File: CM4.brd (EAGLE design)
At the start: 116.8 x 61.4 mm, 7 parts, among them J1 MAGJACK, J2 67800-5001, J3 RASPBERRYPI-40-PIN-GPIO_PTH_N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, J4 67800-5001, J5 67800-5001, J6 67800-5001

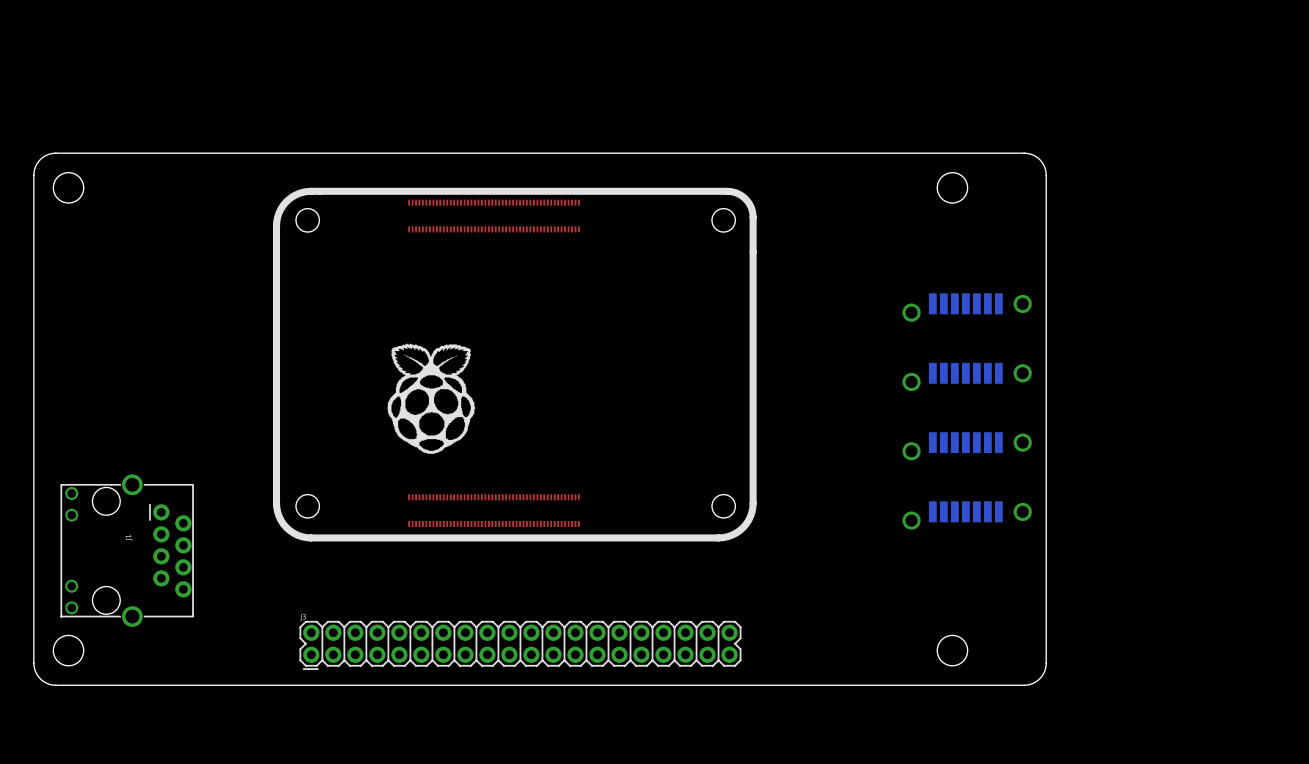
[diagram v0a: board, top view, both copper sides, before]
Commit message: finished board
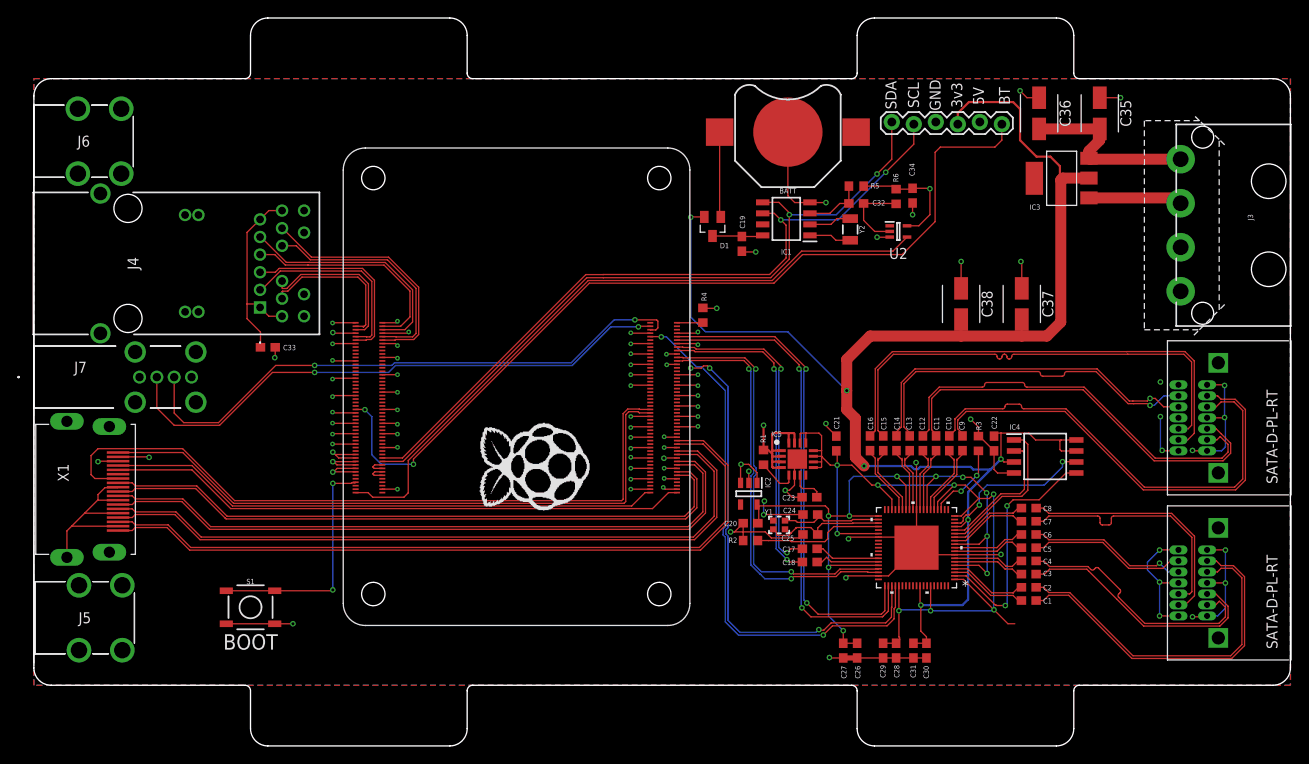
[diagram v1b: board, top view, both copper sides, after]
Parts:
- removed J2: 67800-5001, SamacSys_Parts:67800-5005_2
- added BATT: (no value), SparkFun-Batteries:BATTCON_12MM
- added C1, C10, C11, C12, C13, C14, C15, C16, C17, C18, C19, C2, C22, C3, C32, C33, C34, C4, C5, C6, C7, C8, C9: 0.1uF, SparkFun-Capacitors:0603
- added C20, C26, C28, C30: 1uF, SparkFun-Capacitors:0603
- added C21: 4.7uF, SparkFun-Capacitors:0603
- added C23: 10nF, SparkFun-Capacitors:0603
- added C24, C25: 18pF, SparkFun-Capacitors:0603
- added C27, C29, C31: 2.2uF, SparkFun-Capacitors:0603
- added C35, C36, C37, C38: 865080640004, SamacSys_Parts:865080640004
- added D1: BAT54C, diode:SOT23
- added IC1: PCF85063AT_AAZ, SamacSys_Parts:SOIC127P600X175-8N
- added IC2: MIC5504-1.8YM5-TR, SamacSys_Parts:SOT95P280X145-5N
- added IC3: REG1117, burr-brown:SOT223
- added IC4: W25X40CLSSIG, SamacSys_Parts:SOIC127P790X216-8N
- added IC5: ADP1740ACPZ-1.0-R7, SamacSys_Parts:QFN65P400X400X80-17N
- added J7: KUSBXHT-SLAS1N-O-HRF, SamacSys_Parts:KUSBXHTSLAS1NOHRF
- added R1: 100k, rcl:R0603
- added R2: 6.04k, rcl:R0603
- added R3, R4: 10K, rcl:R0603
- added R5: 510k, rcl:R0603
- added R6: 510K, rcl:R0603
- added S1: MOMENTARY-SWITCH-SPST-SMD-5.2-REDUNDANT, SparkFun-Switches:TACTILE_SWITCH_SMD_5.2MM
- added U$2, U$3: SATA-D-PL-RT, SamacSys_Parts:RIGHTANGLE2PORTSATA
- added U1: 88SE9215A1-NAA2C000, MarvellSATA:QFN76_9X9_MTG
- added U2: 74LVC1G07SE-7, SamacSys_Parts:SOT65P210X110-5N
- added X1: HDMI, raspberrypi_cm:HDMI
- added Y1: 25MHz, SparkFun-Clocks:CRYSTAL-SMD-2.0X1.6MM
- added Y2: 32.768kHz, SparkFun-Clocks:CRYSTAL-SMD-3.2X1.5MM
- J1: value MAGJACK -> (none); device SparkFun-Connectors:MAGJACK -> SparkFun-Connectors:1X06_LOCK
- J3: value RASPBERRYPI-40-PIN-GPIO_PTH_NO_SHROUD -> COMPUTER_PERIPHERAL_POWERRA-VT; device SparkFun-Connectors:2X20 -> SparkFun-Connectors:COMPUTER-PERIPHERAL-POWER-RA-VT
- J4: value 67800-5001 -> 2250508-1; device SamacSys_Parts:67800-5005_2 -> SamacSys_Parts:22505081
- J5, J6: value 67800-5001 -> 8190-3; device SamacSys_Parts:67800-5005_2 -> SamacSys_Parts:81903
- moved J6 119.0 mm to (5.08, 59.0), flipped to the top
- moved J3 114.2 mm to (134.9, 53.1), turned to 270 degrees
- moved J5 112.6 mm to (5.21, 4.05), flipped to the top
- moved J1 110.0 mm to (99.0, 65.0), turned to 0 degrees
- moved J4 90.6 mm to (26.1, 43.6), flipped to the top, turned to 270 degrees
- moved U$1 22.9 mm to (72.7, 32.0), turned to 90 degrees
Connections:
- removed net 3.3V: J3.1, J3.17
- removed net 5V: J3.2, J3.4
- removed net 5V-IN: U$1.77, U$1.79, U$1.81, U$1.83, U$1.85, U$1.87
- new net 1.0VDC: C21.1, C28.1, C29.1, IC5.10, IC5.11, IC5.12, IC5.13, IC5.14, IC5.9, U1.1, U1.19, U1.23, U1.36, U1.44, U1.62, U1.71
- new net 1.8VDC: C20.2, C26.1, C27.1, IC2.5, U1.11, U1.26, U1.32, U1.39, U1.5, U1.53
- new net 3V3: C22.2, C30.1, C31.1, C37.1, C38.1, D1.2, IC3.2, IC4.3, IC4.7, IC4.8, J1.4, U1.16, U1.68
- new net 5VDC: C34.2, C35.1, C36.1, IC2.1, IC2.3, IC3.3, IC5.1, IC5.15, IC5.16, IC5.2, IC5.3, IC5.4, J1.5, J3.5V, J7.1, R1.2, R5.2, R6.2, U$1.77, U$1.79, U$1.81, U$1.83, U$1.85, U$1.87, U2.5, X1.18
- new net AVDD1: U1.48
- new net BUTTON: J1.6, U$1.51
- new net GLOBAL_EN: U$1.99, U2.4
- new net HDMI_CK_N: U$1.190, X1.12
- new net HDMI_CK_P: U$1.188, X1.10
- new net HDMI_D0_N: U$1.184, X1.9
- new net HDMI_D0_P: U$1.182, X1.7
- new net HDMI_D1_N: U$1.178, X1.6
- new net HDMI_D1_P: U$1.176, X1.4
- new net HDMI_D2_N: U$1.172, X1.3
- new net HDMI_D2_P: U$1.170, X1.1
- new net N$1: C23.1, IC5.7
- new net N$10: U$1.199, X1.16
- new net N$11: U$1.153, X1.19
- new net N$12: U$1.151, X1.13
- new net N$13: IC1.1, Y2.P$2
- new net N$14: IC1.2, Y2.P$1
- new net N$16: C32.2, R6.1, U2.2
- new net N$18: J7.2, U$1.103
- new net N$19: J7.3, U$1.105
- new net N$24: BATT.PWR@1, D1.1
- new net N$25: C19.1, D1.3, IC1.8
- new net N$3: IC5.5, R1.1
- new net N$4: C24.2, U1.40, Y1.1
- new net N$5: C25.2, U1.41, Y1.3
- new net N$6: C33.1, J4.1, J4.12, J4.6, J4.7
- new net N$67: R3.2, U1.22
- new net N$68: U1.60
- new net N$69: R4.2, U$1.102
- new net N$7: S1.1, S1.2, U$1.93
- new net N$8: R2.2, U1.42
- new net N$9: U$1.200, X1.15
- new net NRTC_INT: C32.1, IC1.3, R5.1
- new net PCIERXCAP_N: C18.2, U$1.118
- new net PCIERXCAP_P: C17.2, U$1.116
- new net PCIERX_N: C18.1, U1.52
- new net PCIERX_P: C17.1, U1.51
- new net PCIETX_N: U$1.124, U1.55
- new net PCIETX_P: U$1.122, U1.54
- new net PCIE_CLK_N: U$1.110, U1.58
- new net PCIE_CLK_P: U$1.112, U1.59
- new net PCIE_RST: U$1.109, U1.61
- new net RX0_N: C14.2, U1.31
- new net RX0_P: C13.2, U1.30
- new net RX1_N: C10.2, U1.25
- new net RX1_P: C9.2, U1.24
- new net RX2_N: C6.2, U1.10
- new net RX2_P: C5.2, U1.9
- new net RX3_N: C2.2, U1.4
- new net RX3_P: C1.2, U1.3
- new net SATA1RX_N: C15.1, U$2.1_3
- new net SATA1RX_P: C16.1, U$2.1_2
- new net SATA1TX_N: C14.1, U$2.1_5
- new net SATA1TX_P: C13.1, U$2.1_6
- new net SATA1_GND: U$2.1_1, U$2.1_4, U$2.1_7
- new net SATA2RX_N: C11.1, U$2.2_3
- new net SATA2RX_P: C12.1, U$2.2_2
- new net SATA2TX_N: C10.1, U$2.2_5
- new net SATA2TX_P: C9.1, U$2.2_6
- new net SATA2_GND: U$2.2_1, U$2.2_4, U$2.2_7
- new net SATA3RX_N: C7.1, U$3.1_3
- new net SATA3RX_P: C8.1, U$3.1_2
- new net SATA3TX_N: C6.1, U$3.1_5
- new net SATA3TX_P: C5.1, U$3.1_6
- new net SATA3_GND: U$3.1_1, U$3.1_4, U$3.1_7
- new net SATA4RX_N: C3.1, U$3.2_3
- new net SATA4RX_P: C4.1, U$3.2_2
- new net SATA4TX_N: C2.1, U$3.2_5
- new net SATA4TX_P: C1.1, U$3.2_6
- new net SATA4_GND: U$3.2_1, U$3.2_4, U$3.2_7
- new net SCL: IC1.6, J1.2, U$1.80
- new net SDA: IC1.5, J1.1, U$1.82
- new net SPI_CLK: IC4.6, U1.17
- new net SPI_CS: IC4.1, U1.14
- new net SPI_DI: IC4.2, U1.15
- new net SPI_DO: IC4.5, U1.2
- new net TRD0_N: J4.10, U$1.10
- new net TRD0_P: J4.11, U$1.12
- new net TRD1_N: J4.5, U$1.6
- new net TRD1_P: J4.4, U$1.4
- new net TRD2_N: J4.2, U$1.9
- new net TRD2_P: J4.3, U$1.11
- new net TRD3_N: J4.9, U$1.5
- new net TRD3_P: J4.8, U$1.3
- new net TX0_N: C15.2, U1.33
- new net TX0_P: C16.2, U1.34
- new net TX1_N: C11.2, U1.27
- new net TX1_P: C12.2, U1.28
- new net TX2_N: C7.2, U1.12
- new net TX2_P: C8.2, U1.13
- new net TX3_N: C3.2, U1.6
- new net TX3_P: C4.2, U1.7
- net GND: now also BATT.GND, C19.2, C20.1, C21.2, C22.1, C23.2, C24.1, C25.1, C26.2, C27.2, C28.2, C29.2, C30.2, C31.2, C33.2, C34.1, C35.2, C36.2, C37.2, C38.2, IC1.4, IC2.2, IC3.1, IC4.4, IC5.17, IC5.6, J1.3, J3.GND@1, J3.GND@2, J7.4, R2.1, R3.1, R4.1, S1.3, S1.4, U$1.1, U$1.107, U$1.108, U$1.113, U$1.114, U$1.119, U$1.120, U$1.125, U$1.126, U$1.13, U$1.131, U$1.132, U$1.137, U$1.138, U$1.14, U$1.144, U$1.150, U$1.155, U$1.156, U$1.161, U$1.162, U$1.167, U$1.168, U$1.173, U$1.174, U$1.179, U$1.180, U$1.185, U$1.186, U$1.191, U$1.192, U$1.197, U$1.198, U$1.2, U$1.22, U$1.23, U$1.32, U$1.33, U$1.42, U$1.43, U$1.52, U$1.53, U$1.59, U$1.60, U$1.65, U$1.66, U$1.7, U$1.71, U$1.74, U$1.8, U$1.98, U1.29, U1.45, U1.56, U1.77, U1.8, U2.3, X1.11, X1.17, X1.2, X1.5, X1.8, X1.P$1, X1.P$2, X1.P$3, X1.P$4; no longer J3.14, J3.20, J3.25, J3.30, J3.34, J3.39, J3.6, J3.9
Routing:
- net GND: track 0.00 -> 300.6 mm, vias 0 -> 75
- net 3V3: track 0.00 -> 185.8 mm, vias 0 -> 6
- net 1.0VDC: track 0.00 -> 104.3 mm, vias 0 -> 8
- net BUTTON: track 0.00 -> 102.1 mm, vias 0 -> 2
- net 1.8VDC: track 0.00 -> 87.8 mm, vias 0 -> 10
- net HDMI_D2_P: track 0.00 -> 86.6 mm
- net HDMI_D2_N: track 0.00 -> 85.6 mm
- net SCL: track 0.00 -> 84.5 mm, vias 0 -> 2
- net SDA: track 0.00 -> 84.3 mm, vias 0 -> 2
- net N$12: track 0.00 -> 83.0 mm
- net HDMI_D1_P: track 0.00 -> 82.5 mm
- net HDMI_D1_N: track 0.00 -> 81.4 mm
- net 5VDC: track 0.00 -> 79.3 mm, vias 0 -> 7
- net HDMI_D0_P: track 0.00 -> 78.6 mm
- net GLOBAL_EN: track 0.00 -> 78.5 mm
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- added copper zone on layer 15, net 5VDC
- added copper zone on layer 2, net GND
- added copper zone on layer 16, net N$15
- added copper zone on layer 1, net N$17
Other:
- board size 116.8 x 61.4 mm -> 145 x 84 mm
- board text added: "3v3"
- board text added: "5V"
- board text added: "BOOT"
- board text added: "BT"
- board text added: "GND"
- board text added: "SCL"
- board text added: "SDA"
